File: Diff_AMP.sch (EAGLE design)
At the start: 10 parts, among them IC3 MCP1501T-25E_RW, IC4 NCS21911SN2T1G, IC5 NCS21911SN2T1G

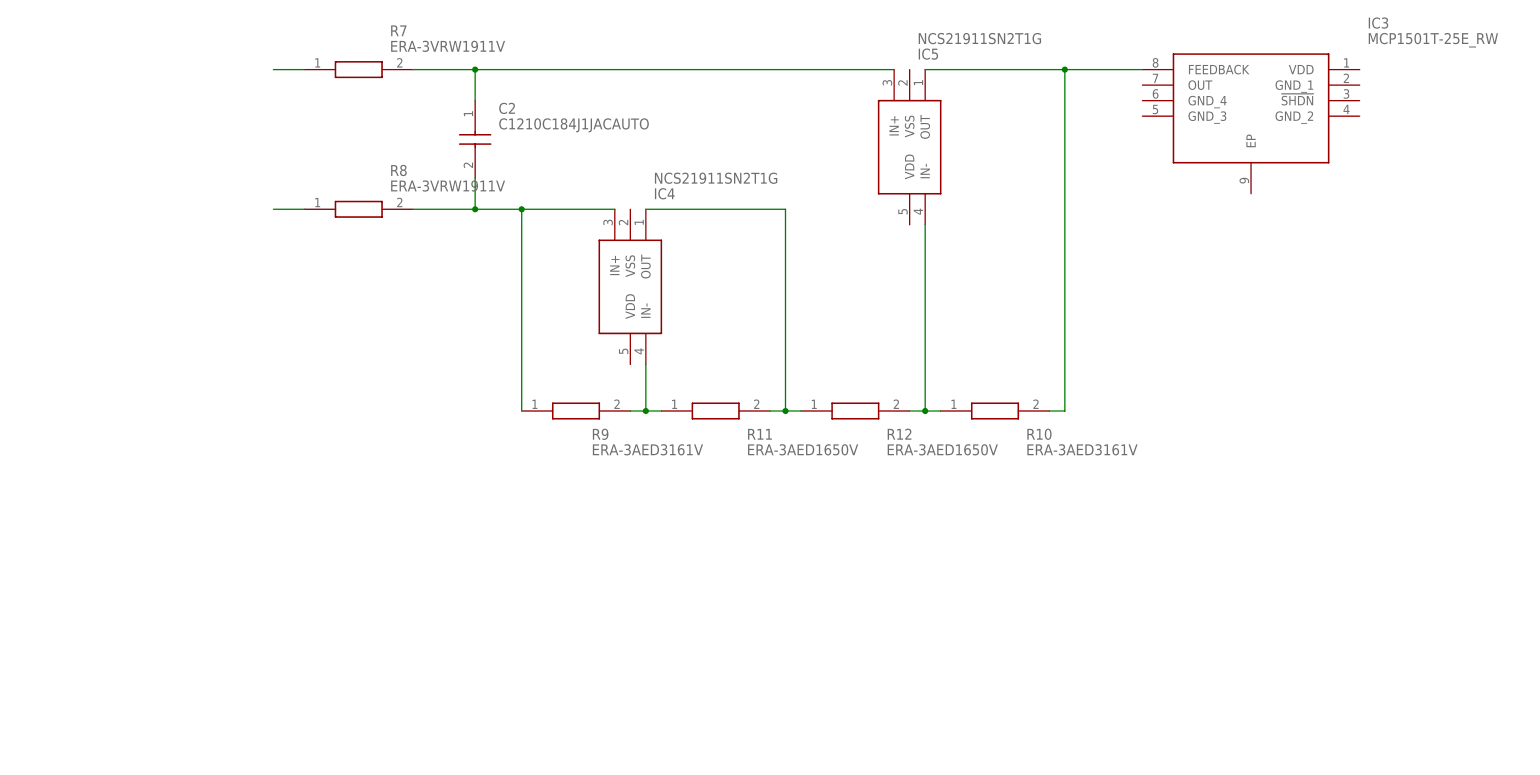
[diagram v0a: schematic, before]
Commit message: board
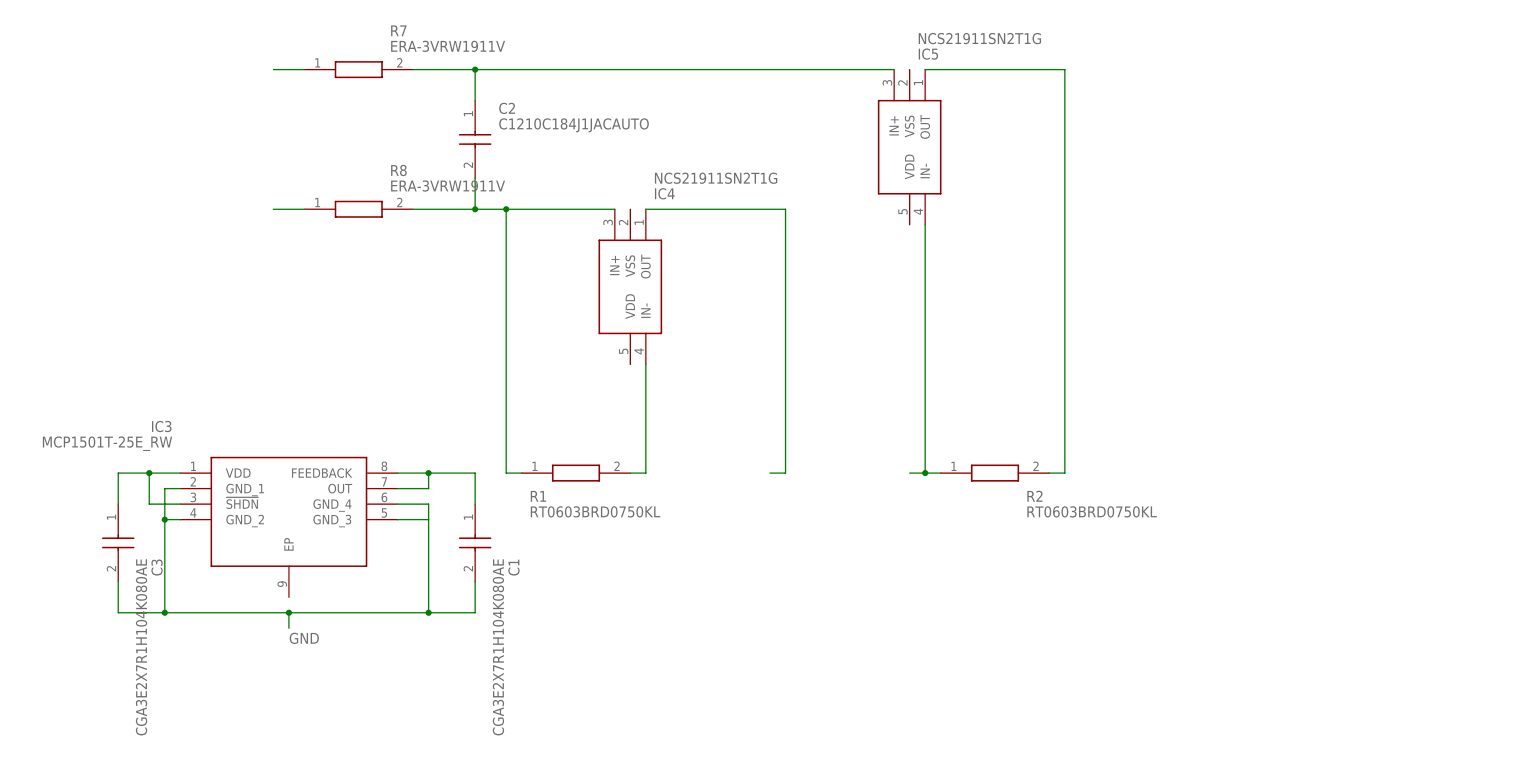
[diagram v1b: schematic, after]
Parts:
- removed R10, R9: ERA-3AED3161V, SamacSys_Parts:ERA-3AED3161V
- removed R11, R12: ERA-3AED1650V, SamacSys_Parts:ERA-3AED1650V
- added C1, C3: CGA3E2X7R1H104K080AE, SamacSys_Parts:CGA3E2X7R1H104K080AE
- added R1, R2: RT0603BRD0750KL, SamacSys_Parts:RT0603BRD0750KL
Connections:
- removed net N$10: C2.2, IC4.IN+, R8.2, R9.1
- new net GND: C1.2, C3.2, IC3.GND_1, IC3.GND_2, IC3.GND_3, IC3.GND_4
- new net N$1: C1.1, IC3.FEEDBACK, IC3.OUT
- new net N$2: C3.1, IC3.!SHDN, IC3.VDD
- new net N$3: C2.2, IC4.IN+, R1.1, R8.2
- net N$11: now also R1.2; no longer R11.1, R9.2
- net N$12: no longer R11.2, R12.1
- net N$13: now also R2.1; no longer R10.1, R12.2
- net N$14: now also R2.2; no longer IC3.FEEDBACK, R10.2
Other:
- moved on the sheet: IC3
